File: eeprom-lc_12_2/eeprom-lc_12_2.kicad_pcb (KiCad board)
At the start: 2 copper layers, 9 parts, among them U5 TXS0108EPW, U6 TXS0108EPW

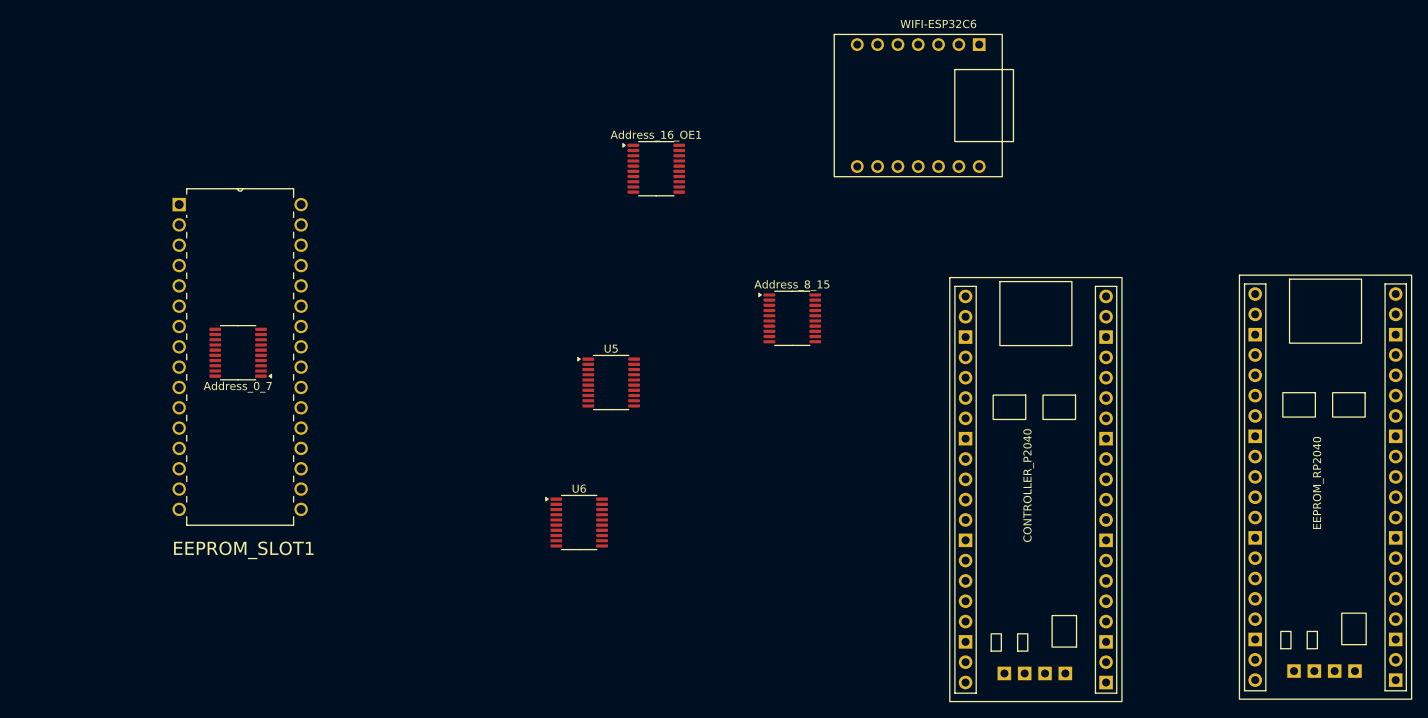
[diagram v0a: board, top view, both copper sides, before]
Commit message: Some work on eeprom code and pcb
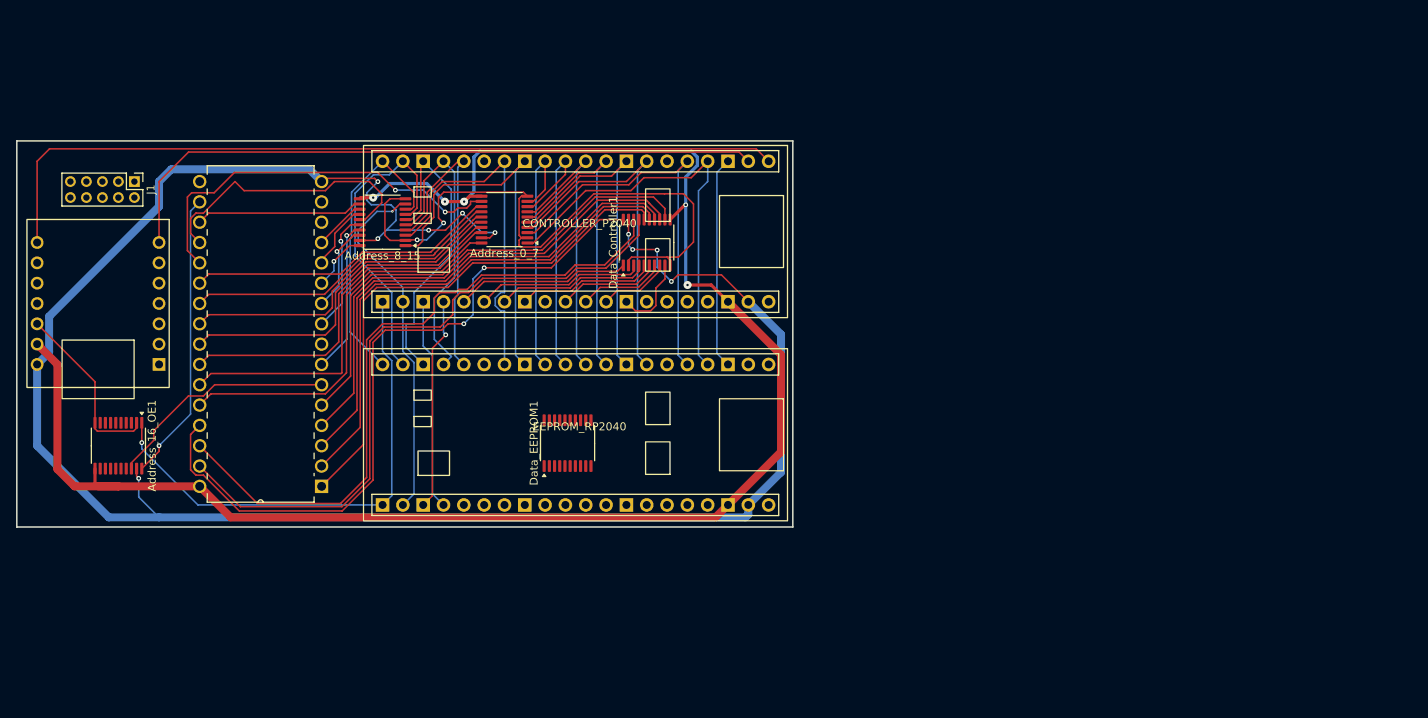
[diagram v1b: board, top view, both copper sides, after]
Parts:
- added J1: Conn_02x05_Pin, Connector_PinHeader_2.00mm:PinHeader_2x05_P2.00mm_Vertical, F.Cu at (90.9, 55.9)
- CONTROLLER_P2040, EEPROM_RP2040: footprint WeAct-rp2040:WeAct-RP2040-Pico -> WeAct-RP2040-Pico:WeAct-RP2040-Pico
- WIFI-ESP32C6: value MOUDLE-SEEEDUINO-XIAO -> WeAct-RP2040-Pico; footprint XIAO-rp2040:MOUDLE14P-2.54-21X17.8MM -> XIAO_PCB:MOUDLE14P-2.54-21X17.8MM
- moved WIFI-ESP32C6 105.5 mm to (86.4, 71.1), turned to -90 degrees
- moved EEPROM_RP2040 94.0 mm to (146.0, 87.5), turned to -90 degrees
- moved Address_16_OE1 75.6 mm to (88.9, 88.9), turned to -90 degrees
- moved CONTROLLER_P2040 66.0 mm to (146.0, 62.1), turned to -90 degrees
- moved Address_8_15 52.6 mm to (121.9, 61.0), turned to 180 degrees
- moved EEPROM_SLOT1 42.9 mm to (99.1, 55.9), turned to 180 degrees
- moved Address_0_7 37.2 mm to (137.2, 60.6)
- moved Data_Controller1 18.1 mm to (154.9, 63.5), turned to 90 degrees
- moved Data_EEPROM1 10.0 mm to (145.0, 88.6), turned to 90 degrees
- renumbered U5 to Data_Controller1, U6 to Data_EEPROM1
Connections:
- Address_0_7 pad 1: unconnected-(Address_0_7-A1-Pad1) -> /A0_3V3
- Address_0_7 pad 10: unconnected-(Address_0_7-OE-Pad10) -> /VCC_3V3
- Address_0_7 pad 3: unconnected-(Address_0_7-A2-Pad3) -> /A1_3V3
- Address_0_7 pad 4: unconnected-(Address_0_7-A3-Pad4) -> /A2_3V3
- Address_0_7 pad 5: unconnected-(Address_0_7-A4-Pad5) -> /A3_3V3
- Address_0_7 pad 6: unconnected-(Address_0_7-A5-Pad6) -> /A4_3V3
- Address_0_7 pad 7: unconnected-(Address_0_7-A6-Pad7) -> /A5_3V3
- Address_0_7 pad 8: unconnected-(Address_0_7-A7-Pad8) -> /A6_3V3
- Address_0_7 pad 9: unconnected-(Address_0_7-A8-Pad9) -> /A7_3V3
- Address_16_OE1 pad 1: unconnected-(Address_16_OE1-A1-Pad1) -> /A16_3V3
- Address_16_OE1 pad 10: unconnected-(Address_16_OE1-OE-Pad10) -> /VCC_3V3
- Address_16_OE1 pad 3: unconnected-(Address_16_OE1-A2-Pad3) -> /OE_3V3
- Address_8_15 pad 1: unconnected-(Address_8_15-A1-Pad1) -> /A8_3V3
- Address_8_15 pad 10: unconnected-(Address_8_15-OE-Pad10) -> /VCC_3V3
- Address_8_15 pad 3: unconnected-(Address_8_15-A2-Pad3) -> /A9_3V3
- Address_8_15 pad 4: unconnected-(Address_8_15-A3-Pad4) -> /A10_3V3
- Address_8_15 pad 5: unconnected-(Address_8_15-A4-Pad5) -> /A11_3V3
- Address_8_15 pad 6: unconnected-(Address_8_15-A5-Pad6) -> /A12_3V3
- Address_8_15 pad 7: unconnected-(Address_8_15-A6-Pad7) -> /A13_3V3
- Address_8_15 pad 8: unconnected-(Address_8_15-A7-Pad8) -> /A14_3V3
- Address_8_15 pad 9: unconnected-(Address_8_15-A8-Pad9) -> /A15_3V3
- CONTROLLER_P2040 pad 1: unconnected-(CONTROLLER_P2040-GP0-Pad1) -> Net-(CONTROLLER_P2040-GP0)
- CONTROLLER_P2040 pad 10: unconnected-(CONTROLLER_P2040-GP8-Pad10) -> /A5_3V3
- CONTROLLER_P2040 pad 11: unconnected-(CONTROLLER_P2040-GP9-Pad11) -> /A6_3V3
- CONTROLLER_P2040 pad 12: unconnected-(CONTROLLER_P2040-GP10-Pad12) -> /A7_3V3
- CONTROLLER_P2040 pad 13: unconnected-(CONTROLLER_P2040-GP11-Pad13) -> /A8_3V3
- CONTROLLER_P2040 pad 14: unconnected-(CONTROLLER_P2040-GP12-Pad14) -> /A9_3V3
- CONTROLLER_P2040 pad 16: unconnected-(CONTROLLER_P2040-GP13-Pad16) -> /A10_3V3
- CONTROLLER_P2040 pad 17: unconnected-(CONTROLLER_P2040-GP14-Pad17) -> /A11_3V3
- CONTROLLER_P2040 pad 18: unconnected-(CONTROLLER_P2040-GP15-Pad18) -> /A12_3V3
- CONTROLLER_P2040 pad 19: unconnected-(CONTROLLER_P2040-GP16-Pad19) -> /A13_3V3
- CONTROLLER_P2040 pad 2: unconnected-(CONTROLLER_P2040-GP1-Pad2) -> Net-(CONTROLLER_P2040-GP1)
- CONTROLLER_P2040 pad 20: unconnected-(CONTROLLER_P2040-GP17-Pad20) -> /A14_3V3
- CONTROLLER_P2040 pad 21: unconnected-(CONTROLLER_P2040-GP18-Pad21) -> /A16_3V3
- CONTROLLER_P2040 pad 22: unconnected-(CONTROLLER_P2040-GP19-Pad22) -> /A15_3V3
- CONTROLLER_P2040 pad 23: unconnected-(CONTROLLER_P2040-GP20-Pad23) -> Net-(CONTROLLER_P2040-GP20)
- CONTROLLER_P2040 pad 24: unconnected-(CONTROLLER_P2040-GP21-Pad24) -> Net-(CONTROLLER_P2040-GP21)
- CONTROLLER_P2040 pad 25: unconnected-(CONTROLLER_P2040-GP22-Pad25) -> /D0_3V3_CO
- CONTROLLER_P2040 pad 26: unconnected-(CONTROLLER_P2040-GP23-Pad26) -> /D1_3V3_CO
- CONTROLLER_P2040 pad 27: unconnected-(CONTROLLER_P2040-GP24-Pad27) -> /D2_3V3_CO
- CONTROLLER_P2040 pad 28: unconnected-(CONTROLLER_P2040-GP25-Pad28) -> /D3_3V3_CO
- CONTROLLER_P2040 pad 3: unconnected-(CONTROLLER_P2040-GP2-Pad3) -> /OE_3V3
- CONTROLLER_P2040 pad 30: unconnected-(CONTROLLER_P2040-GP26-Pad30) -> /D4_3V3_CO
- CONTROLLER_P2040 pad 31: unconnected-(CONTROLLER_P2040-GP27-Pad31) -> /D5_3V3_CO
- CONTROLLER_P2040 pad 32: unconnected-(CONTROLLER_P2040-GP28-Pad32) -> /D6_3V3_CO
- CONTROLLER_P2040 pad 33: unconnected-(CONTROLLER_P2040-GP29-Pad33) -> /D7_3V3_CO
- CONTROLLER_P2040 pad 36: unconnected-(CONTROLLER_P2040-3V3-Pad36) -> /VCC_3V3
- CONTROLLER_P2040 pad 38: unconnected-(CONTROLLER_P2040-GND-Pad38) -> /GND
- CONTROLLER_P2040 pad 39: unconnected-(CONTROLLER_P2040-VIN-Pad39) -> /VCC_5V
- CONTROLLER_P2040 pad 4: unconnected-(CONTROLLER_P2040-GP3-Pad4) -> /A0_3V3
- CONTROLLER_P2040 pad 5: unconnected-(CONTROLLER_P2040-GP4-Pad5) -> /A1_3V3
- CONTROLLER_P2040 pad 7: unconnected-(CONTROLLER_P2040-GP5-Pad7) -> /A2_3V3
- CONTROLLER_P2040 pad 8: unconnected-(CONTROLLER_P2040-GP6-Pad8) -> /A3_3V3
- CONTROLLER_P2040 pad 9: unconnected-(CONTROLLER_P2040-GP7-Pad9) -> /A4_3V3
- Data_Controller1 pad 1: unconnected-(U5-A1-Pad1) -> /D0_3V3_CO
- Data_Controller1 pad 10: unconnected-(U5-OE-Pad10) -> /VCC_3V3
- Data_Controller1 pad 3: unconnected-(U5-A2-Pad3) -> /D1_3V3_CO
- Data_Controller1 pad 4: unconnected-(U5-A3-Pad4) -> /D2_3V3_CO
- Data_Controller1 pad 5: unconnected-(U5-A4-Pad5) -> /D3_3V3_CO
- Data_Controller1 pad 6: unconnected-(U5-A5-Pad6) -> /D4_3V3_CO
- Data_Controller1 pad 7: unconnected-(U5-A6-Pad7) -> /D5_3V3_CO
- Data_Controller1 pad 8: unconnected-(U5-A7-Pad8) -> /D6_3V3_CO
- Data_Controller1 pad 9: unconnected-(U5-A8-Pad9) -> /D7_3V3_CO
- Data_EEPROM1 pad 1: unconnected-(U6-A1-Pad1) -> /D0_3V3_EE
- Data_EEPROM1 pad 10: unconnected-(U6-OE-Pad10) -> /OE_Data
- Data_EEPROM1 pad 3: unconnected-(U6-A2-Pad3) -> /D1_3V3_EE
- Data_EEPROM1 pad 4: unconnected-(U6-A3-Pad4) -> /D2_3V3_EE
- Data_EEPROM1 pad 5: unconnected-(U6-A4-Pad5) -> /D3_3V3_EE
- Data_EEPROM1 pad 6: unconnected-(U6-A5-Pad6) -> /D4_3V3_EE
- Data_EEPROM1 pad 7: unconnected-(U6-A6-Pad7) -> /D5_3V3_EE
- Data_EEPROM1 pad 8: unconnected-(U6-A7-Pad8) -> /D6_3V3_EE
- Data_EEPROM1 pad 9: unconnected-(U6-A8-Pad9) -> /D7_3V3_EE
- EEPROM_RP2040 pad 1: unconnected-(EEPROM_RP2040-GP0-Pad1) -> /OE_Data
- EEPROM_RP2040 pad 10: unconnected-(EEPROM_RP2040-GP8-Pad10) -> /A5_3V3
- EEPROM_RP2040 pad 11: unconnected-(EEPROM_RP2040-GP9-Pad11) -> /A6_3V3
- EEPROM_RP2040 pad 12: unconnected-(EEPROM_RP2040-GP10-Pad12) -> /A7_3V3
- EEPROM_RP2040 pad 13: unconnected-(EEPROM_RP2040-GP11-Pad13) -> /A8_3V3
- EEPROM_RP2040 pad 14: unconnected-(EEPROM_RP2040-GP12-Pad14) -> /A9_3V3
- EEPROM_RP2040 pad 16: unconnected-(EEPROM_RP2040-GP13-Pad16) -> /A10_3V3
- EEPROM_RP2040 pad 17: unconnected-(EEPROM_RP2040-GP14-Pad17) -> /A11_3V3
- EEPROM_RP2040 pad 18: unconnected-(EEPROM_RP2040-GP15-Pad18) -> /A12_3V3
- EEPROM_RP2040 pad 19: unconnected-(EEPROM_RP2040-GP16-Pad19) -> /A13_3V3
- EEPROM_RP2040 pad 20: unconnected-(EEPROM_RP2040-GP17-Pad20) -> /A14_3V3
- EEPROM_RP2040 pad 21: unconnected-(EEPROM_RP2040-GP18-Pad21) -> /A16_3V3
- EEPROM_RP2040 pad 22: unconnected-(EEPROM_RP2040-GP19-Pad22) -> /A15_3V3
- EEPROM_RP2040 pad 23: unconnected-(EEPROM_RP2040-GP20-Pad23) -> Net-(CONTROLLER_P2040-GP21)
- EEPROM_RP2040 pad 24: unconnected-(EEPROM_RP2040-GP21-Pad24) -> Net-(CONTROLLER_P2040-GP20)
- EEPROM_RP2040 pad 25: unconnected-(EEPROM_RP2040-GP22-Pad25) -> /D0_3V3_EE
- EEPROM_RP2040 pad 26: unconnected-(EEPROM_RP2040-GP23-Pad26) -> /D1_3V3_EE
- EEPROM_RP2040 pad 27: unconnected-(EEPROM_RP2040-GP24-Pad27) -> /D2_3V3_EE
- EEPROM_RP2040 pad 28: unconnected-(EEPROM_RP2040-GP25-Pad28) -> /D3_3V3_EE
- EEPROM_RP2040 pad 3: unconnected-(EEPROM_RP2040-GP2-Pad3) -> /OE_3V3
- EEPROM_RP2040 pad 30: unconnected-(EEPROM_RP2040-GP26-Pad30) -> /D4_3V3_EE
- EEPROM_RP2040 pad 31: unconnected-(EEPROM_RP2040-GP27-Pad31) -> /D5_3V3_EE
- EEPROM_RP2040 pad 32: unconnected-(EEPROM_RP2040-GP28-Pad32) -> /D6_3V3_EE
- EEPROM_RP2040 pad 33: unconnected-(EEPROM_RP2040-GP29-Pad33) -> /D7_3V3_EE
- EEPROM_RP2040 pad 36: unconnected-(EEPROM_RP2040-3V3-Pad36) -> /VCC_3V3
- EEPROM_RP2040 pad 38: unconnected-(EEPROM_RP2040-GND-Pad38) -> /GND
- EEPROM_RP2040 pad 39: unconnected-(EEPROM_RP2040-VIN-Pad39) -> /VCC_5V
- EEPROM_RP2040 pad 4: unconnected-(EEPROM_RP2040-GP3-Pad4) -> /A0_3V3
- EEPROM_RP2040 pad 5: unconnected-(EEPROM_RP2040-GP4-Pad5) -> /A1_3V3
- EEPROM_RP2040 pad 7: unconnected-(EEPROM_RP2040-GP5-Pad7) -> /A2_3V3
- EEPROM_RP2040 pad 8: unconnected-(EEPROM_RP2040-GP6-Pad8) -> /A3_3V3
- EEPROM_RP2040 pad 9: unconnected-(EEPROM_RP2040-GP7-Pad9) -> /A4_3V3
- EEPROM_SLOT1 pad 1: /VCC_5V -> unconnected-(EEPROM_SLOT1-VPP-Pad1)
- EEPROM_SLOT1 pad 24: /GND -> unconnected-(EEPROM_SLOT1-~G-Pad24)
- EEPROM_SLOT1 pad 31: /VCC_5V -> unconnected-(EEPROM_SLOT1-~P-Pad31)
- WIFI-ESP32C6 pad 1: unconnected-(WIFI-ESP32C6-PA02_A0_D0-Pad1) -> Net-(J1-Pin_1)
- WIFI-ESP32C6 pad 10: unconnected-(WIFI-ESP32C6-PA5_A9_D9_MISO-Pad10) -> Net-(J1-Pin_8)
- WIFI-ESP32C6 pad 11: unconnected-(WIFI-ESP32C6-PA6_A10_D10_MOSI-Pad11) -> Net-(J1-Pin_9)
- WIFI-ESP32C6 pad 12: unconnected-(WIFI-ESP32C6-3V3-Pad12) -> /VCC_3V3
- WIFI-ESP32C6 pad 2: unconnected-(WIFI-ESP32C6-PA4_A1_D1-Pad2) -> Net-(J1-Pin_2)
- WIFI-ESP32C6 pad 3: unconnected-(WIFI-ESP32C6-PA10_A2_D2-Pad3) -> Net-(J1-Pin_3)
- WIFI-ESP32C6 pad 4: unconnected-(WIFI-ESP32C6-PA11_A3_D3-Pad4) -> Net-(J1-Pin_4)
- WIFI-ESP32C6 pad 5: unconnected-(WIFI-ESP32C6-PA8_A4_D4_SDA-Pad5) -> Net-(J1-Pin_5)
- WIFI-ESP32C6 pad 6: unconnected-(WIFI-ESP32C6-PA9_A5_D5_SCL-Pad6) -> Net-(J1-Pin_6)
- WIFI-ESP32C6 pad 7: unconnected-(WIFI-ESP32C6-PB08_A6_D6_TX-Pad7) -> Net-(CONTROLLER_P2040-GP1)
- WIFI-ESP32C6 pad 8: unconnected-(WIFI-ESP32C6-PB09_A7_D7_RX-Pad8) -> Net-(CONTROLLER_P2040-GP0)
- WIFI-ESP32C6 pad 9: unconnected-(WIFI-ESP32C6-PA7_A8_D8_SCK-Pad9) -> Net-(J1-Pin_7)
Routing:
- net /VCC_5V: track 0.00 -> 252.7 mm, vias 0 -> 10
- net /GND: track 0.00 -> 216.7 mm, vias 0 -> 5
- net Net-(CONTROLLER_P2040-GP0): track 0.00 -> 102.9 mm
- net /VCC_3V3: track 0.00 -> 101.4 mm, vias 0 -> 2
- net /D0_5V: track 0.00 -> 90.0 mm, vias 0 -> 2
- net /D1_5V: track 0.00 -> 84.3 mm
- net /D2_5V: track 0.00 -> 84.2 mm
- net Net-(CONTROLLER_P2040-GP1): track 0.00 -> 83.3 mm
- net /D3_5V: track 0.00 -> 66.2 mm
- net /D4_5V: track 0.00 -> 64.9 mm
- net /D5_5V: track 0.00 -> 63.6 mm
- net /A16_3V3: track 0.00 -> 62.8 mm, vias 0 -> 1
- net /D6_5V: track 0.00 -> 62.4 mm
- net /D7_5V: track 0.00 -> 61.6 mm
- net /A0_3V3: track 0.00 -> 53.1 mm
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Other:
- board outline added: 97 x 48.3 mm
